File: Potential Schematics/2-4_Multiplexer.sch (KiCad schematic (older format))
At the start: 18 parts

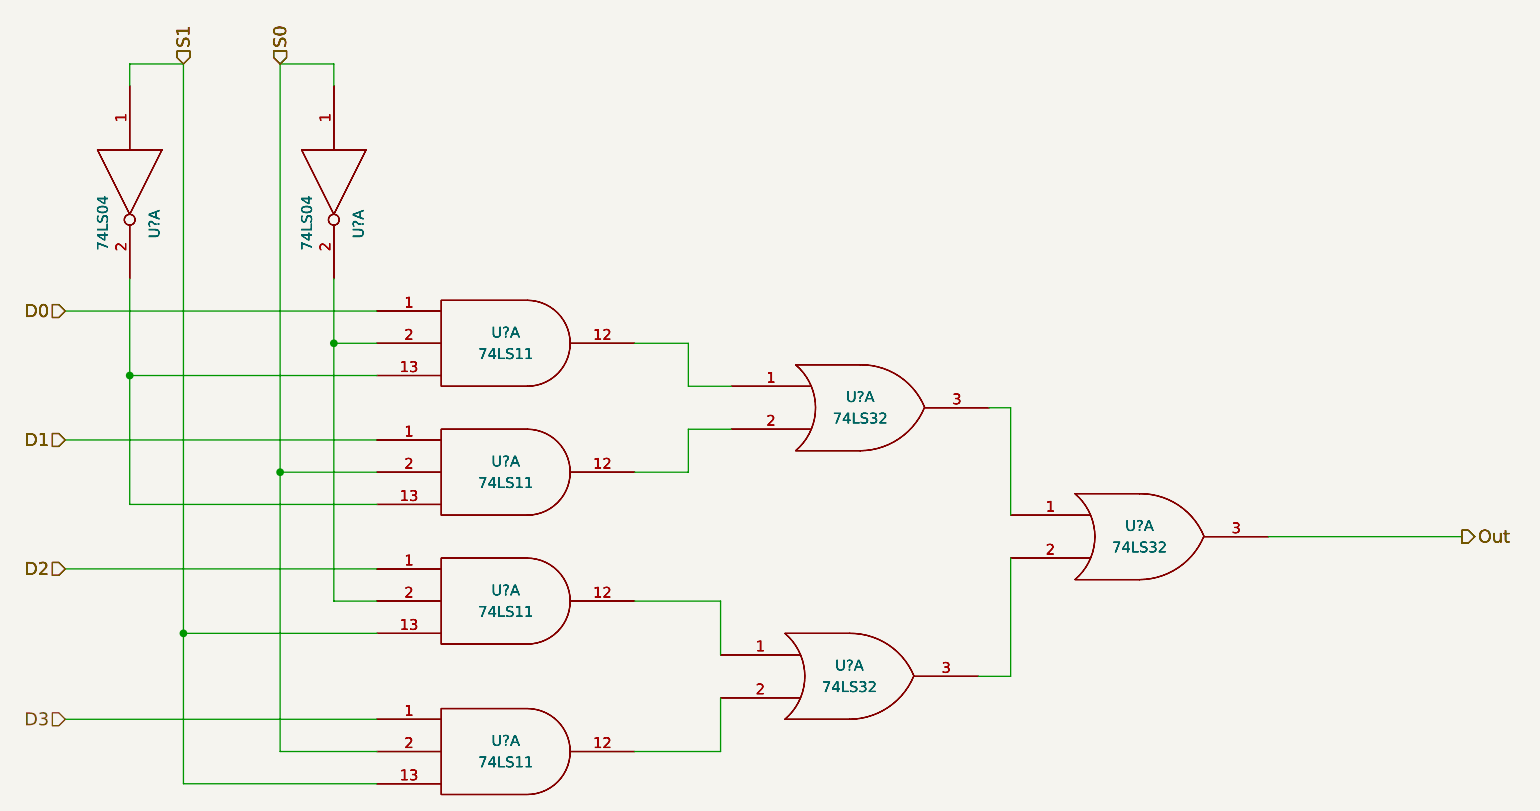
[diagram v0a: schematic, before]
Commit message: Made Full ALU
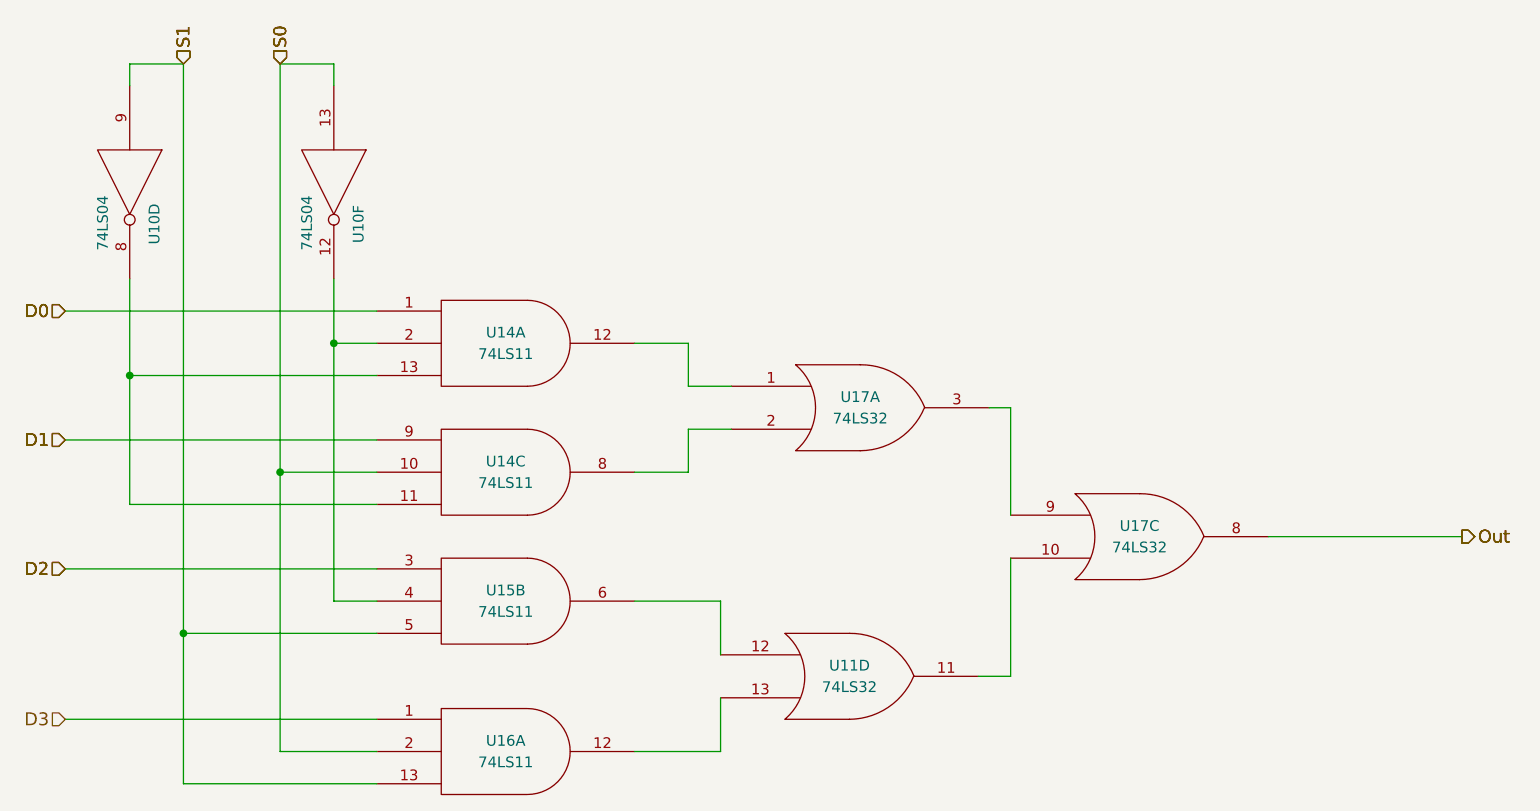
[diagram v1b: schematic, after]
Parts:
- removed U? (x3): 74LS32, symbol 74LS32
- removed U? (x4): 74LS11, symbol 74LS11
- removed U? (x2): 74LS04, symbol 74LS04
- gave numbers to parts that had none: 6
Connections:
- net D1: now also U7.9; no longer U7.1
- net D2: now also U7.3; no longer U7.1
- net Out: now also U9.8; no longer U9.3
- net S0: now also U1.13, U7.10; no longer U1.1, U7.2
- net S1: now also U1.9, U7.5; no longer U1.1, U7.13
- net at U9.2: now also U7.8; no longer U7.12
- net at U9.3: now also U9.9; no longer U9.1
- net at U8.12: now also U3.13; no longer U3.2
- new net: U3.11, U9.10
- new net: U3.12, U7.6
- new net: U1.8, U6.13, U7.11
- new net: U1.12, U6.2, U7.4
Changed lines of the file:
@@
 $Descr A4 11693 8268
 encoding utf-8
-Sheet 6 6
-Title ""
+Sheet 10 22
+Title "2:4_Multiplexer"
 Date ""
 Rev "1"
@@
 S1
 $Comp
-L 74LS32 U?
+L 74LS32 U9
 U 1 1 5B98E2FD
 P 6700 3500
-F 0 "U?" H 6700 3550 50  0000 C CNN
+AR Path="/5B990C59/5B990C5E/5B98E051/5B98E2FD" Ref="U9"  Part="1"
+AR Path="/5B990C59/5B99BC00/5B98E051/5B98E2FD" Ref="U17"  Part="1"
+AR Path="/5B990C59/5B99C896/5B98E051/5B98E2FD" Ref="U24"  Part="1"
+AR Path="/5B990C59/5B99C8B8/5B98E051/5B98E2FD" Ref="U32"  Part="1"
+F 0 "U17" H 6700 3550 50  0000 C CNN
 F 1 "74LS32" H 6700 3450 50  0000 C CNN
 F 2 "" H 6700 3500 50  0001 C CNN
@@
 	1    0    0    -1
 $EndComp
-$Comp
-L 74LS32 U?
-U 1 1 5B98E304
-P 6650 4750
-F 0 "U?" H 6650 4800 50  0000 C CNN
-F 1 "74LS32" H 6650 4700 50  0000 C CNN
-F 2 "" H 6650 4750 50  0001 C CNN
-F 3 "" H 6650 4750 50  0001 C CNN
-	1    6650 4750
-	1    0    0    -1
-$EndComp
 Text HLabel 9500 4100 2    60   Output ~ 0
 Out
@@
 Wire Wire Line
 	5900 3600 6100 3600
-$Comp
-L 74LS11 U?
-U 1 1 5B98E312
-P 5050 3200
-F 0 "U?" H 5050 3250 50  0000 C CNN
-F 1 "74LS11" H 5050 3150 50  0000 C CNN
-F 2 "" H 5050 3200 50  0001 C CNN
-F 3 "" H 5050 3200 50  0001 C CNN
-	1    5050 3200
-	1    0    0    -1
-$EndComp
-$Comp
-L 74LS11 U?
-U 1 1 5B98E319
-P 5050 3800
-F 0 "U?" H 5050 3850 50  0000 C CNN
-F 1 "74LS11" H 5050 3750 50  0000 C CNN
-F 2 "" H 5050 3800 50  0001 C CNN
-F 3 "" H 5050 3800 50  0001 C CNN
-	1    5050 3800
-	1    0    0    -1
-$EndComp
-$Comp
-L 74LS11 U?
-U 1 1 5B98E320
-P 5050 4400
-F 0 "U?" H 5050 4450 50  0000 C CNN
-F 1 "74LS11" H 5050 4350 50  0000 C CNN
-F 2 "" H 5050 4400 50  0001 C CNN
-F 3 "" H 5050 4400 50  0001 C CNN
-	1    5050 4400
-	1    0    0    -1
-$EndComp
-$Comp
-L 74LS04 U?
-U 1 1 5B98E327
-P 4250 2450
-F 0 "U?" H 4445 2565 50  0000 C CNN
-F 1 "74LS04" H 4440 2325 50  0000 C CNN
-F 2 "" H 4250 2450 50  0001 C CNN
-F 3 "" H 4250 2450 50  0001 C CNN
-	1    4250 2450
-	0    1    1    0
-$EndComp
-$Comp
-L 74LS04 U?
-U 1 1 5B98E32E
-P 3300 2450
-F 0 "U?" H 3495 2565 50  0000 C CNN
-F 1 "74LS04" H 3490 2325 50  0000 C CNN
-F 2 "" H 3300 2450 50  0001 C CNN
-F 3 "" H 3300 2450 50  0001 C CNN
-	1    3300 2450
-	0    1    1    0
-$EndComp
 Wire Wire Line
 	3000 3050 4450 3050
@@
 S1
 $Comp
-L 74LS32 U?
-U 1 1 5B98E34D
-P 6700 3500
-F 0 "U?" H 6700 3550 50  0000 C CNN
-F 1 "74LS32" H 6700 3450 50  0000 C CNN
-F 2 "" H 6700 3500 50  0001 C CNN
-F 3 "" H 6700 3500 50  0001 C CNN
-	1    6700 3500
-	1    0    0    -1
-$EndComp
-$Comp
-L 74LS32 U?
-U 1 1 5B98E354
+L 74LS32 U3
+U 4 1 5B98E354
 P 6650 4750
-F 0 "U?" H 6650 4800 50  0000 C CNN
+AR Path="/5B990C59/5B990C5E/5B98E051/5B98E354" Ref="U3"  Part="4"
+AR Path="/5B990C59/5B99BC00/5B98E051/5B98E354" Ref="U11"  Part="4"
+AR Path="/5B990C59/5B99C896/5B98E051/5B98E354" Ref="U19"  Part="4"
+AR Path="/5B990C59/5B99C8B8/5B98E051/5B98E354" Ref="U26"  Part="4"
+F 0 "U11" H 6650 4800 50  0000 C CNN
 F 1 "74LS32" H 6650 4700 50  0000 C CNN
 F 2 "" H 6650 4750 50  0001 C CNN
 F 3 "" H 6650 4750 50  0001 C CNN
-	1    6650 4750
+	4    6650 4750
 	1    0    0    -1
 $EndComp
@@
 Out
 $Comp
-L 74LS11 U?
+L 74LS11 U6
 U 1 1 5B98E35C
 P 5050 3200
-F 0 "U?" H 5050 3250 50  0000 C CNN
+AR Path="/5B990C59/5B990C5E/5B98E051/5B98E35C" Ref="U6"  Part="2"
+AR Path="/5B990C59/5B99BC00/5B98E051/5B98E35C" Ref="U14"  Part="1"
+AR Path="/5B990C59/5B99C896/5B98E051/5B98E35C" Ref="U16"  Part="3"
+AR Path="/5B990C59/5B99C8B8/5B98E051/5B98E35C" Ref="U29"  Part="2"
+F 0 "U14" H 5050 3250 50  0000 C CNN
 F 1 "74LS11" H 5050 3150 50  0000 C CNN
 F 2 "" H 5050 3200 50  0001 C CNN
@@
 $EndComp
 $Comp
-L 74LS11 U?
-U 1 1 5B98E363
+L 74LS11 U7
+U 3 1 5B98E363
 P 5050 3800
-F 0 "U?" H 5050 3850 50  0000 C CNN
+AR Path="/5B990C59/5B990C5E/5B98E051/5B98E363" Ref="U7"  Part="1"
+AR Path="/5B990C59/5B99BC00/5B98E051/5B98E363" Ref="U14"  Part="3"
+AR Path="/5B990C59/5B99C896/5B98E051/5B98E363" Ref="U22"  Part="2"
+AR Path="/5B990C59/5B99C8B8/5B98E051/5B98E363" Ref="U30"  Part="1"
+F 0 "U14" H 5050 3850 50  0000 C CNN
 F 1 "74LS11" H 5050 3750 50  0000 C CNN
 F 2 "" H 5050 3800 50  0001 C CNN
 F 3 "" H 5050 3800 50  0001 C CNN
-	1    5050 3800
-	1    0    0    -1
-$EndComp
-$Comp
-L 74LS11 U?
-U 1 1 5B98E36A
+	3    5050 3800
+	1    0    0    -1
+$EndComp
+$Comp
+L 74LS11 U7
+U 2 1 5B98E36A
 P 5050 4400
-F 0 "U?" H 5050 4450 50  0000 C CNN
+AR Path="/5B990C59/5B990C5E/5B98E051/5B98E36A" Ref="U7"  Part="3"
+AR Path="/5B990C59/5B99BC00/5B98E051/5B98E36A" Ref="U15"  Part="2"
+AR Path="/5B990C59/5B99C896/5B98E051/5B98E36A" Ref="U23"  Part="1"
+AR Path="/5B990C59/5B99C8B8/5B98E051/5B98E36A" Ref="U30"  Part="3"
+F 0 "U15" H 5050 4450 50  0000 C CNN
 F 1 "74LS11" H 5050 4350 50  0000 C CNN
 F 2 "" H 5050 4400 50  0001 C CNN
 F 3 "" H 5050 4400 50  0001 C CNN
-	1    5050 4400
-	1    0    0    -1
-$EndComp
-$Comp
-L 74LS04 U?
-U 1 1 5B98E371
+	2    5050 4400
+	1    0    0    -1
+$EndComp
+$Comp
+L 74LS04 U1
+U 6 1 5B98E371
 P 4250 2450
-F 0 "U?" H 4445 2565 50  0000 C CNN
+AR Path="/5B990C59/5B990C5E/5B98E051/5B98E371" Ref="U1"  Part="6"
+AR Path="/5B990C59/5B99BC00/5B98E051/5B98E371" Ref="U10"  Part="6"
+AR Path="/5B990C59/5B99C896/5B98E051/5B98E371" Ref="U18"  Part="6"
+AR Path="/5B990C59/5B99C8B8/5B98E051/5B98E371" Ref="U25"  Part="6"
+F 0 "U10" H 4445 2565 50  0000 C CNN
 F 1 "74LS04" H 4440 2325 50  0000 C CNN
 F 2 "" H 4250 2450 50  0001 C CNN
 F 3 "" H 4250 2450 50  0001 C CNN
-	1    4250 2450
+	6    4250 2450
 	0    1    1    0
 $EndComp
 $Comp
-L 74LS04 U?
-U 1 1 5B98E378
+L 74LS04 U1
+U 4 1 5B98E378
 P 3300 2450
-F 0 "U?" H 3495 2565 50  0000 C CNN
+AR Path="/5B990C59/5B990C5E/5B98E051/5B98E378" Ref="U1"  Part="4"
+AR Path="/5B990C59/5B99BC00/5B98E051/5B98E378" Ref="U10"  Part="4"
+AR Path="/5B990C59/5B99C896/5B98E051/5B98E378" Ref="U18"  Part="4"
+AR Path="/5B990C59/5B99C8B8/5B98E051/5B98E378" Ref="U25"  Part="4"
+F 0 "U10" H 3495 2565 50  0000 C CNN
 F 1 "74LS04" H 3490 2325 50  0000 C CNN
 F 2 "" H 3300 2450 50  0001 C CNN
 F 3 "" H 3300 2450 50  0001 C CNN
-	1    3300 2450
+	4    3300 2450
 	0    1    1    0
 $EndComp
 $Comp
-L 74LS11 U?
-U 1 1 5B98E37F
+L 74LS11 U8
+U 1 1 5B98E386
 P 5050 5100
-F 0 "U?" H 5050 5150 50  0000 C CNN
+AR Path="/5B990C59/5B990C5E/5B98E051/5B98E386" Ref="U8"  Part="2"
+AR Path="/5B990C59/5B99BC00/5B98E051/5B98E386" Ref="U16"  Part="1"
+AR Path="/5B990C59/5B99C896/5B98E051/5B98E386" Ref="U23"  Part="3"
+AR Path="/5B990C59/5B99C8B8/5B98E051/5B98E386" Ref="U31"  Part="2"
+F 0 "U16" H 5050 5150 50  0000 C CNN
 F 1 "74LS11" H 5050 5050 50  0000 C CNN
 F 2 "" H 5050 5100 50  0001 C CNN
@@
 	1    0    0    -1
 $EndComp
-$Comp
-L 74LS11 U?
-U 1 1 5B98E386
-P 5050 5100
-F 0 "U?" H 5050 5150 50  0000 C CNN
-F 1 "74LS11" H 5050 5050 50  0000 C CNN
-F 2 "" H 5050 5100 50  0001 C CNN
-F 3 "" H 5050 5100 50  0001 C CNN
-	1    5050 5100
-	1    0    0    -1
-$EndComp
 Wire Wire Line
 	6050 5100 6050 4850
@@
 Connection ~ 4000 3800
 $Comp
-L 74LS32 U?
-U 1 1 5B98E397
+L 74LS32 U9
+U 3 1 5B98E397
 P 8000 4100
-F 0 "U?" H 8000 4150 50  0000 C CNN
+AR Path="/5B990C59/5B990C5E/5B98E051/5B98E397" Ref="U9"  Part="3"
+AR Path="/5B990C59/5B99BC00/5B98E051/5B98E397" Ref="U17"  Part="3"
+AR Path="/5B990C59/5B99C896/5B98E051/5B98E397" Ref="U24"  Part="3"
+AR Path="/5B990C59/5B99C8B8/5B98E051/5B98E397" Ref="U32"  Part="3"
+F 0 "U17" H 8000 4150 50  0000 C CNN
 F 1 "74LS32" H 8000 4050 50  0000 C CNN
 F 2 "" H 8000 4100 50  0001 C CNN
 F 3 "" H 8000 4100 50  0001 C CNN
-	1    8000 4100
-	1    0    0    -1
-$EndComp
-$Comp
-L 74LS32 U?
-U 1 1 5B98E39E
-P 8000 4100
-F 0 "U?" H 8000 4150 50  0000 C CNN
-F 1 "74LS32" H 8000 4050 50  0000 C CNN
-F 2 "" H 8000 4100 50  0001 C CNN
-F 3 "" H 8000 4100 50  0001 C CNN
-	1    8000 4100
-	1    0    0    -1
-$EndComp
+	3    8000 4100
+	1    0    0    -1
+$EndComp
